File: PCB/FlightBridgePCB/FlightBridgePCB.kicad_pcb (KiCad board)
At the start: 2 copper layers, 65 x 35 mm, 12 parts, among them J1 Raspberry_Pi_2_3, J2 AVR-ISP-6, U1 ATmega128A-AU, Y1 Crystal

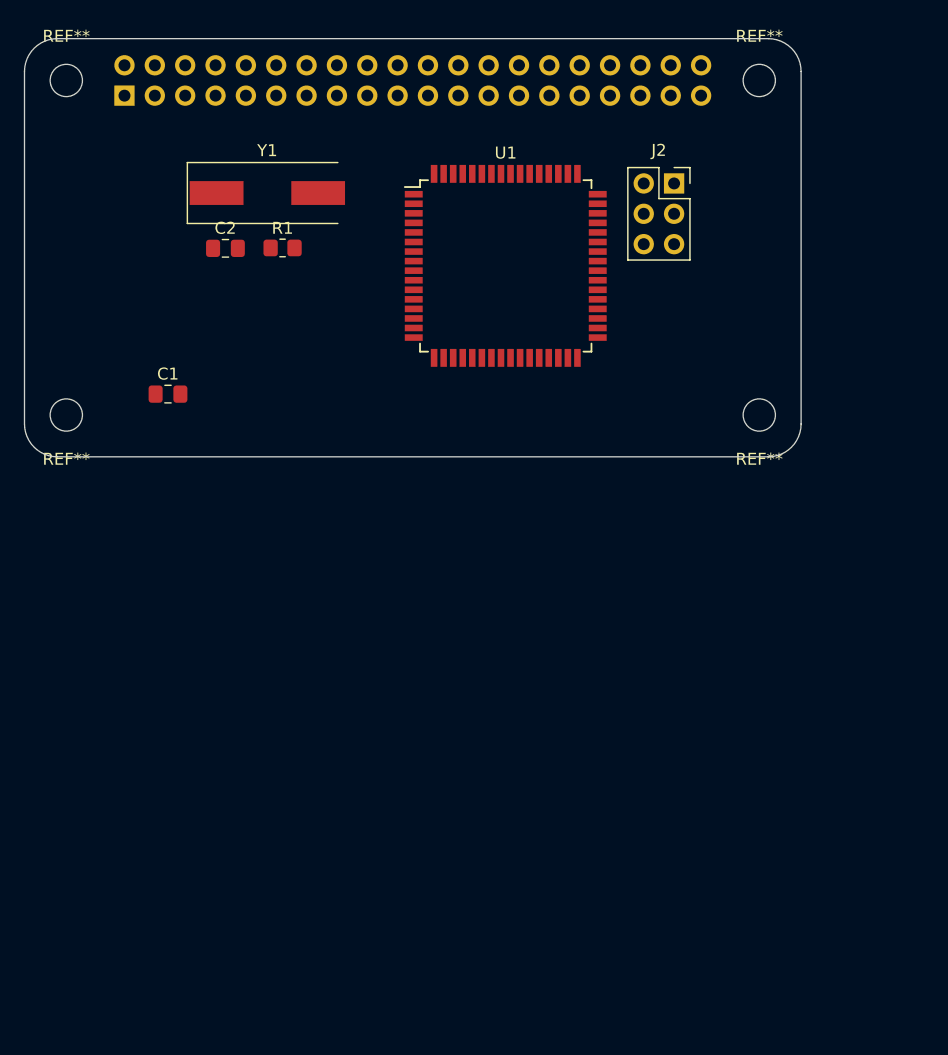
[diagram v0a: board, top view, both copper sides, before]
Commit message: PCB Update
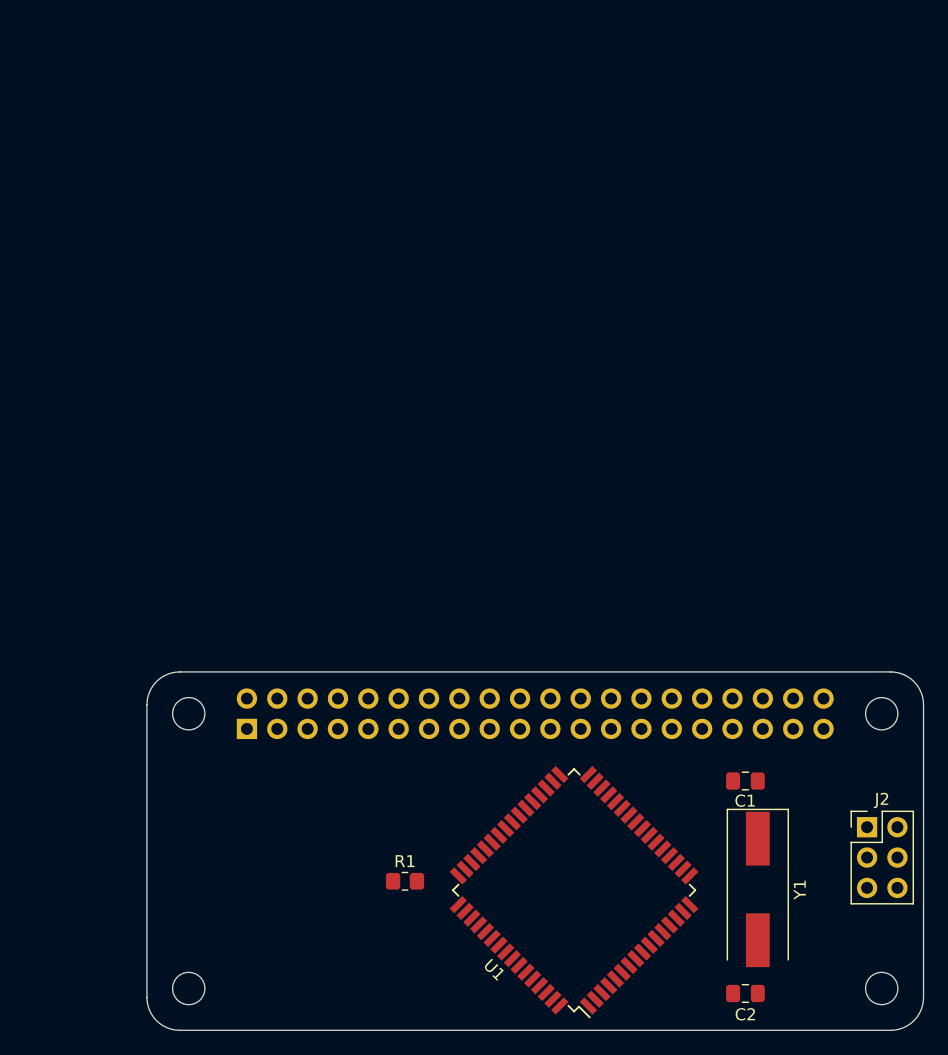
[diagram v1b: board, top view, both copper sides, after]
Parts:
- removed the REF** at (161.5, 46.5)
- removed the REF** at (161.5, 18.5)
- removed the REF** at (103.5, 46.5)
- removed the REF** at (103.5, 18.5)
- added REF**: MountingHole_2.7mm_M2.5, MountingHole:MountingHole_2.7mm_M2.5, F.Cu at (171.7, 94.5)
- added REF**: MountingHole_2.7mm_M2.5, MountingHole:MountingHole_2.7mm_M2.5, F.Cu at (171.7, 71.5)
- added REF**: MountingHole_2.7mm_M2.5, MountingHole:MountingHole_2.7mm_M2.5, F.Cu at (113.7, 94.5)
- added REF**: MountingHole_2.7mm_M2.5, MountingHole:MountingHole_2.7mm_M2.5, F.Cu at (113.7, 71.5)
- J2: footprint Connector_PinSocket_2.54mm:PinSocket_2x03_P2.54mm_Vertical -> Connector_PinHeader_2.54mm:PinHeader_2x03_P2.54mm_Vertical
- moved C2 76.1 mm to (160.3, 94.9)
- moved Y1 71.3 mm to (161.4, 86.2), turned to 270 degrees
- moved C1 58.2 mm to (160.3, 77.1), turned to 180 degrees
- moved J2 56.2 mm to (170.5, 81.0)
- moved ? 54.0 mm to (126.7, 81.3)
- moved J1 54.0 mm to (118.6, 72.8)
- moved R1 54.0 mm to (131.8, 85.5)
- moved U1 52.6 mm to (146.0, 86.3), turned to 135 degrees
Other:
- board size 65 x 35 mm -> 65 x 30 mm
